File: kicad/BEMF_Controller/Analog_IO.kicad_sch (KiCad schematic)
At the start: 30 parts, among them J4 HEADER6, U10 OPA2376AIDR, U7 OPA2376AIDR, U9 OPA2376AIDR

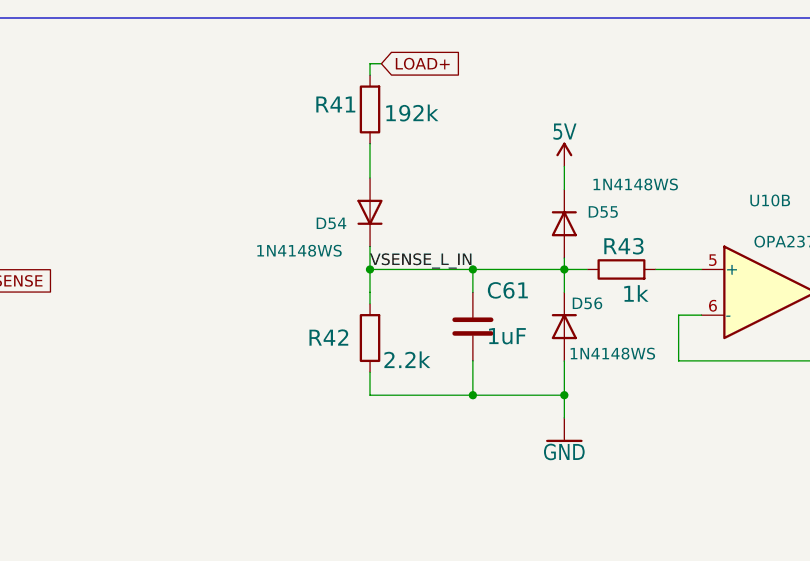
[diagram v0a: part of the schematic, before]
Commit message: Pretty much complete, but a few things left to do.
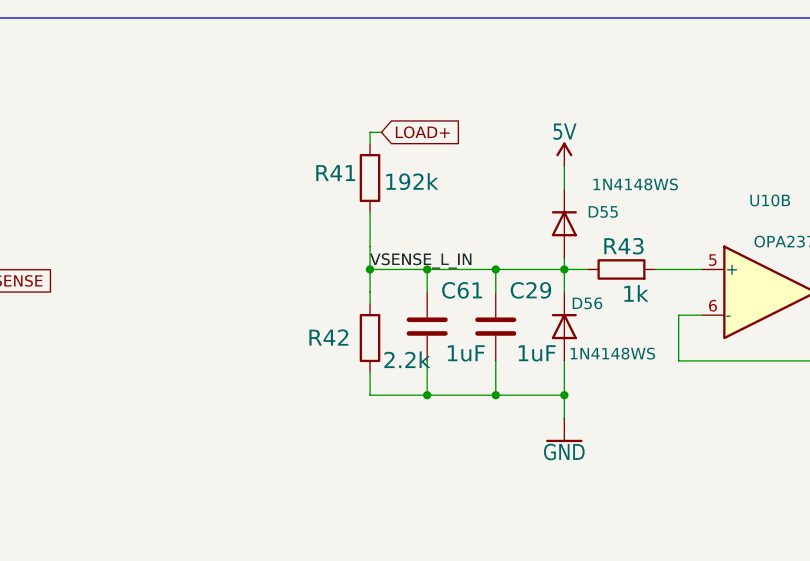
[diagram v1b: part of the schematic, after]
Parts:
- removed D54: 1N4148WS, Diode_SMD:D_SOD-323, symbol Diode:1N4148WS
- added C29: 1uF, Capacitor_SMD:C_1812_4532Metric, symbol Component_Library:CHV1812N250105MXT
- J4: footprint main:6PINVALULOK -> TerminalBlock_Phoenix:TerminalBlock_Phoenix_MKDS-1,5-6_1x06_P5.00mm_Horizontal
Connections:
- net GND: now also C29.2
- net VSENSE_L_IN: now also R41.1, C29.1
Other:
- moved on the sheet: C61, R41
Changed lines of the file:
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@@
 	)
 	(junction
-		(at 110.49 43.18)
+		(at 105.41 43.18)
 		(diameter 0)
 		(color 0 0 0 0)
 	)
 	(junction
-		(at 99.06 29.21)
+		(at 105.41 29.21)
 		(diameter 0)
 		(color 0 0 0 0)
 	)
 	(junction
-		(at 110.49 29.21)
+		(at 99.06 29.21)
 		(diameter 0)
 		(color 0 0 0 0)
@@
 	)
 	(junction
+		(at 113.03 29.21)
+		(diameter 0)
+		(color 0 0 0 0)
+	)
+	(junction
 		(at 151.13 91.44)
 		(diameter 0)
@@
 	)
 	(junction
+		(at 113.03 43.18)
+		(diameter 0)
+		(color 0 0 0 0)
+	)
+	(junction
 		(at 120.65 129.54)
 		(diameter 0)
@@
 	(wire
 		(pts
-			(xy 99.06 29.21) (xy 110.49 29.21)
+			(xy 99.06 29.21) (xy 105.41 29.21)
 		)
 		(stroke
@@
 	(wire
 		(pts
-			(xy 110.49 31.75) (xy 110.49 29.21)
+			(xy 105.41 31.75) (xy 105.41 29.21)
 		)
 		(stroke
@@
 	(wire
 		(pts
-			(xy 110.49 43.18) (xy 99.06 43.18)
+			(xy 105.41 43.18) (xy 113.03 43.18)
 		)
 		(stroke
@@
 	(wire
 		(pts
+			(xy 105.41 43.18) (xy 99.06 43.18)
+		)
+		(stroke
+			(width 0)
+			(type default)
+		)
+	)
+	(wire
+		(pts
 			(xy 34.29 128.27) (xy 34.29 130.81)
 		)
@@
 	(wire
 		(pts
-			(xy 99.06 6.35) (xy 99.06 7.62)
+			(xy 99.06 13.97) (xy 99.06 15.24)
 		)
 		(stroke
@@
 	(wire
 		(pts
-			(xy 110.49 43.18) (xy 120.65 43.18)
-		)
-		(stroke
-			(width 0)
-			(type default)
-		)
-	)
-	(wire
-		(pts
 			(xy 110.49 88.9) (xy 120.65 88.9)
 		)
@@
 	(wire
 		(pts
-			(xy 110.49 29.21) (xy 120.65 29.21)
+			(xy 182.88 125.73) (xy 182.88 123.19)
 		)
 		(stroke
@@
 	(wire
 		(pts
-			(xy 182.88 125.73) (xy 182.88 123.19)
+			(xy 120.65 39.37) (xy 120.65 43.18)
 		)
 		(stroke
@@
 	(wire
 		(pts
-			(xy 120.65 39.37) (xy 120.65 43.18)
+			(xy 113.03 29.21) (xy 120.65 29.21)
 		)
 		(stroke
@@
 	(wire
 		(pts
+			(xy 113.03 43.18) (xy 120.65 43.18)
+		)
+		(stroke
+			(width 0)
+			(type default)
+		)
+	)
+	(wire
+		(pts
 			(xy 63.5 130.81) (xy 66.04 130.81)
 		)
@@
 	(wire
 		(pts
-			(xy 99.06 6.35) (xy 100.33 6.35)
+			(xy 99.06 13.97) (xy 100.33 13.97)
+		)
+		(stroke
+			(width 0)
+			(type default)
+		)
+	)
+	(wire
+		(pts
+			(xy 113.03 29.21) (xy 113.03 31.75)
 		)
 		(stroke
@@
 	(wire
 		(pts
-			(xy 99.06 15.24) (xy 99.06 19.05)
+			(xy 99.06 22.86) (xy 99.06 26.67)
 		)
 		(stroke
@@
 	(wire
 		(pts
+			(xy 113.03 39.37) (xy 113.03 43.18)
+		)
+		(stroke
+			(width 0)
+			(type default)
+		)
+	)
+	(wire
+		(pts
 			(xy 24.13 87.63) (xy 34.29 87.63)
 		)
@@
 	(wire
 		(pts
-			(xy 110.49 39.37) (xy 110.49 43.18)
+			(xy 105.41 39.37) (xy 105.41 43.18)
+		)
+		(stroke
+			(width 0)
+			(type default)
+		)
+	)
+	(wire
+		(pts
+			(xy 105.41 29.21) (xy 113.03 29.21)
 		)
 		(stroke
@@
 	(global_label "LOAD+"
 		(shape input)
-		(at 100.33 6.35 0)
+		(at 100.33 13.97 0)
 		(fields_autoplaced yes)
 		(effects
@@
 		)
 		(property "Intersheetrefs" "${INTERSHEET_REFS}"
-			(at 109.6048 6.35 0)
+			(at 109.6048 13.97 0)
 			(effects
 				(font
@@
 	(symbol
 		(lib_id "Component_Library:R192k")
-		(at 99.06 11.43 180)
+		(at 99.06 19.05 180)
 		(unit 1)
 		(exclude_from_sim no)
@@
 		(dnp no)
 		(property "Reference" "R41"
-			(at 95.25 9.906 0)
+			(at 95.25 17.526 0)
 			(effects
 				(font
@@
 		)
 		(property "Value" "192k"
-			(at 103.632 12.954 0)
+			(at 103.632 20.574 0)
 			(effects
 				(font
@@
 		)
 		(property "Footprint" "Resistor_SMD:R_1206_3216Metric"
-			(at 100.838 11.43 90)
+			(at 100.838 19.05 90)
 			(effects
 				(font
@@
 		)
 		(property "Datasheet" "~"
-			(at 99.06 11.43 0)
+			(at 99.06 19.05 0)
 			(effects
 				(font
@@
 		)
 		(property "Description" "Resistor"
-			(at 99.06 11.43 0)
+			(at 99.06 19.05 0)
 			(effects
 				(font
@@
 	(symbol
 		(lib_id "Component_Library:CHV1812N250105MXT")
-		(at 110.49 35.56 0)
+		(at 105.41 35.56 0)
 		(unit 1)
 		(exclude_from_sim no)
@@
 		(dnp no)
 		(property "Reference" "C61"
-			(at 112.014 32.639 0)
+			(at 106.934 32.639 0)
 			(effects
 				(font
@@
 		)
 		(property "Value" "1uF"
-			(at 112.014 37.719 0)
+			(at 107.442 39.624 0)
 			(effects
 				(font
@@
 		)
 		(property "Footprint" "Capacitor_SMD:C_1812_4532Metric"
-			(at 111.4552 39.37 0)
+			(at 106.3752 39.37 0)
 			(effects
 				(font
@@
 		)
 		(property "Datasheet" "https://88ce57.p3cdn1.secureserver.net/wp-content/uploads/2023/01/chv_series-1.pdf"
-			(at 110.49 35.56 0)
+			(at 105.41 35.56 0)
 			(effects
 				(font
@@
 		)
 		(property "Description" "HVCAP1812 X7R 1UF 20% 250V"
-			(at 110.49 35.56 0)
+			(at 105.41 35.56 0)
 			(effects
 				(font
@@
 	)
 	(symbol
-		(lib_id "Diode:1N4148WS")
-		(at 99.06 22.86 90)
-		(unit 1)
-		(exclude_from_sim no)
-		(in_bom yes)
-		(on_board yes)
-		(dnp no)
-		(property "Reference" "D54"
-			(at 96.52 24.1301 90)
-			(effects
-				(font
-					(size 1.27 1.27)
-				)
-				(justify left)
-			)
-		)
-		(property "Value" "1N4148WS"
-			(at 96.012 27.178 90)
-			(effects
-				(font
-					(size 1.27 1.27)
-				)
-				(justify left)
-			)
-		)
-		(property "Footprint" "Diode_SMD:D_SOD-323"
-			(at 103.505 22.86 0)
-			(effects
-				(font
-					(size 1.27 1.27)
-				)
-				(hide yes)
-			)
-		)
-		(property "Datasheet" "https://www.vishay.com/docs/85751/1n4148ws.pdf"
-			(at 99.06 22.86 0)
-			(effects
-				(font
-					(size 1.27 1.27)
-				)
-				(hide yes)
-			)
-		)
-		(property "Description" "75V 0.15A Fast switching Diode, SOD-323"
-			(at 99.06 22.86 0)
-			(effects
-				(font
-					(size 1.27 1.27)
-				)
-				(hide yes)
-			)
-		)
-		(property "Sim.Device" "D"
-			(at 99.06 22.86 0)
-			(effects
-				(font
-					(size 1.27 1.27)
-				)
-				(hide yes)
-			)
-		)
-		(property "Sim.Pins" "1=K 2=A"
-			(at 99.06 22.86 0)
-			(effects
-				(font
-					(size 1.27 1.27)
-				)
-				(hide yes)
-			)
-		)
-		(pin "1"
-		)
-		(pin "2"
-		)
-		(instances
-			(project "BEMF_Controller"
-				(path "/80a514a6-29a9-4699-8a7d-cff678a7ed07/6990bf25-70eb-45d9-b265-2461b625100e"
-					(reference "D54")
-					(unit 1)
-				)
-			)
-		)
-	)
-	(symbol
 		(lib_id "Component_Library:R1k")
 		(at 40.64 87.63 90)
@@
 			)
 		)
-		(property "Footprint" "main:6PINVALULOK"
+		(property "Footprint" "TerminalBlock_Phoenix:TerminalBlock_Phoenix_MKDS-1,5-6_1x06_P5.00mm_Horizontal"
 			(at 19.05 165.1 0)
 			(effects
@@
 					(unit 1)
 				)
+			)
+		)
+	)
+	(symbol
+		(lib_id "Component_Library:CHV1812N250105MXT")
+		(at 113.03 35.56 0)
+		(unit 1)
+		(exclude_from_sim no)
+		(in_bom yes)
+		(on_board yes)
+		(dnp no)
+		(property "Reference" "C29"
+			(at 114.554 32.639 0)
+			(effects
+				(font
+					(size 1.778 1.778)
+				)
+				(justify left bottom)
+			)
+		)
+		(property "Value" "1uF"
+			(at 115.316 39.624 0)
+			(effects
+				(font
+					(size 1.778 1.778)
+				)
+				(justify left bottom)
+			)
+		)
+		(property "Footprint" "Capacitor_SMD:C_1812_4532Metric"
+			(at 113.9952 39.37 0)
+			(effects
+				(font
+					(size 1.27 1.27)
+				)
+				(hide yes)
+			)
+		)
+		(property "Datasheet" "https://88ce57.p3cdn1.secureserver.net/wp-content/uploads/2023/01/chv_series-1.pdf"
+			(at 113.03 35.56 0)
+			(effects
+				(font
+					(size 1.27 1.27)
+				)
+				(hide yes)
+			)
+		)
+		(property "Description" "HVCAP1812 X7R 1UF 20% 250V"
+			(at 113.03 35.56 0)
+			(effects
+				(font
+					(size 1.27 1.27)
+				)
+				(hide yes)
+			)
+		)
+		(pin "1"
+		)
+		(pin "2"
+		)
+		(instances
+			(project "MEG_Controller"
+				(path "/80a514a6-29a9-4699-8a7d-cff678a7ed07/6990bf25-70eb-45d9-b265-2461b625100e"
+					(reference "C29")
+					(unit 1)
+				)
